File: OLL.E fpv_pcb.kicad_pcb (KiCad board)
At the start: 6 copper layers, 47.6 x 41.5 mm, 134 parts, among them J1 Micro_SD_Card, J10 Conn_01x05_Pin, J2 RC, J8 reciver, J9 TYPE-C-31-M-12, M1 M1 front left, M2 M2 front right, M3 M3 rear right, M4 m4 rear left, Q1 2N7002, Q2 SUD45P03-09, SW1 SW_SPST, SW2 SW_SPST, U1 MP2315GJ, U10 AON7410, U11 UCC27511ADBV, U12 AON7410, U13 BMP280, U14 STM32H753VITx, U15 USBLC6-2SC6, U3 MP2315GJ, U4 ICM-42688-P, U5 UCC27511ADBV, U6 ul_AON7410, U7 UCC27511ADBV, U8 AON7410, U9 UCC27511ADBV, Y2 8HMz

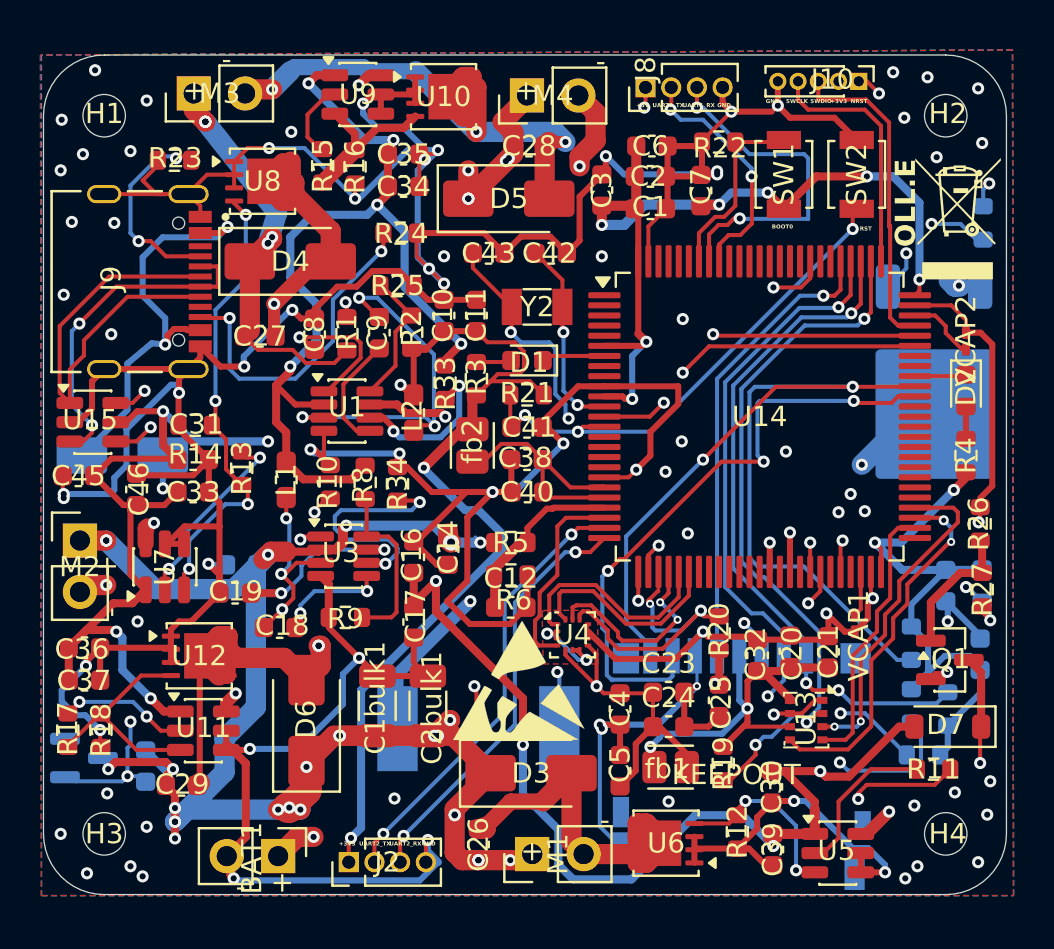
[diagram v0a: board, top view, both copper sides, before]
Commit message: latest scemetic
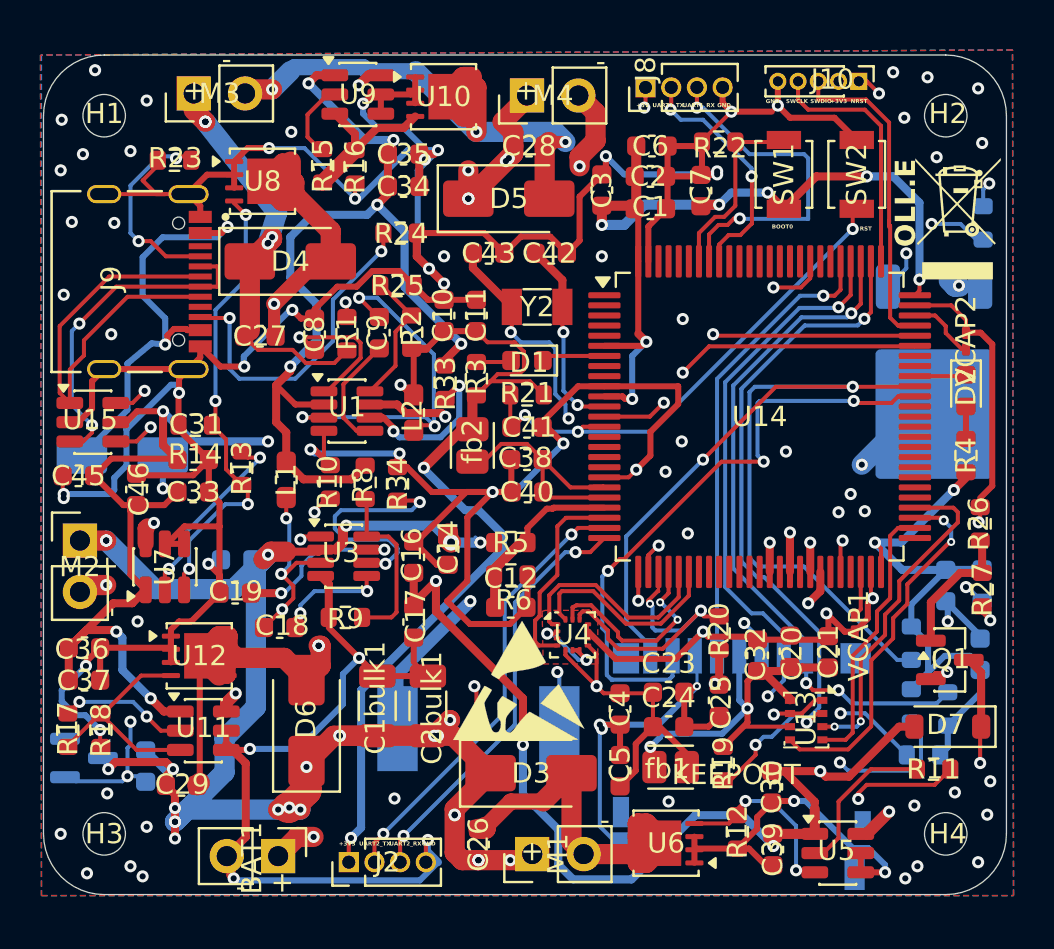
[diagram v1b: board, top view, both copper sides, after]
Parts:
- moved C15 0.35 mm to (142.9, 97.2)
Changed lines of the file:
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@@
 	(footprint "Capacitor_SMD:C_0603_1608Metric"
 		(layer "B.Cu")
-		(at 143.2 97.4 180)
+		(at 142.95 97.15 180)
 		(descr "Capacitor SMD 0603 (1608 Metric), square (rectangular) end terminal, IPC-7351 nominal, (Body size source: IPC-SM-782 page 76, https://www.pcb-3d.com/wordpress/wp-content/uploads/ipc-sm-782a_amendment_1_and_2.pdf), generated with kicad-footprint-generator")
 		(tags "capacitor")
@@
 		(start 151.85 81)
 		(end 151.85 82.15)
-		(width 0.2)
+		(width 0.4)
 		(layer "F.Cu")
 		(net 1)
@@
 		(start 141.15 79.655)
 		(end 140.57 79.075)
-		(width 0.2)
+		(width 0.3)
 		(layer "F.Cu")
 		(net 1)
@@
 		(start 142.825 77.465)
 		(end 143.49 76.8)
-		(width 0.2)
+		(width 0.3)
 		(layer "F.Cu")
 		(net 1)
@@
 		(start 151.85 82.15)
 		(end 153.2 83.5)
-		(width 0.2)
+		(width 0.4)
 		(layer "F.Cu")
 		(net 1)
@@
 		(start 143.49 76.8)
 		(end 144.55 76.8)
-		(width 0.2)
+		(width 0.3)
 		(layer "F.Cu")
 		(net 1)
@@
 		(start 141.15 80.2)
 		(end 141.15 79.655)
-		(width 0.2)
+		(width 0.3)
 		(layer "F.Cu")
 		(net 1)
@@
 		(start 140.57 79.03)
 		(end 141.485 78.115)
-		(width 0.2)
+		(width 0.3)
 		(layer "F.Cu")
 		(net 1)
@@
 	)
 	(segment
+		(start 173.8 112.6)
+		(end 175 112.6)
+		(width 0.3)
+		(layer "F.Cu")
+		(net 1)
+	)
+	(segment
 		(start 141.575 93.8)
 		(end 141.575 92.2)
@@
 		(start 142.825 77.465)
 		(end 142.825 78.765)
-		(width 0.2)
+		(width 0.3)
 		(layer "F.Cu")
 		(net 1)
@@
 		(start 151.975 77.1)
 		(end 152.7 77.1)
-		(width 0.2)
+		(width 0.4)
 		(layer "F.Cu")
 		(net 1)
@@
 	)
 	(segment
-		(start 173.8 112.6)
-		(end 175 112.6)
-		(width 0.3)
-		(layer "F.Cu")
-		(net 1)
-	)
-	(segment
 		(start 151.375 92.575)
 		(end 152.6 93.8)
@@
 		(start 164.175 79.8)
 		(end 163.3 80.675)
-		(width 0.2)
+		(width 0.3)
 		(layer "F.Cu")
 		(net 1)
@@
 	)
 	(segment
+		(start 163.3 82.4)
+		(end 163.3 80.675)
+		(width 0.3)
+		(layer "F.Cu")
+		(net 1)
+	)
+	(segment
 		(start 167.7 111.425)
 		(end 168.275 111.425)
@@
 	)
 	(segment
-		(start 163.3 80.675)
-		(end 163.3 82.4)
-		(width 0.2)
-		(layer "F.Cu")
-		(net 1)
-	)
-	(segment
 		(start 134.7 90.35)
 		(end 135.053052 90.35)
@@
 		(start 151.975 77.1)
 		(end 151.975 78.7)
-		(width 0.2)
+		(width 0.4)
 		(layer "F.Cu")
 		(net 1)
@@
 		(start 141.485 78.115)
 		(end 142.825 78.115)
-		(width 0.2)
+		(width 0.3)
 		(layer "F.Cu")
 		(net 1)
@@
 	)
 	(segment
-		(start 141.6 97.4)
-		(end 141.55 97.35)
-		(width 0.3)
-		(layer "B.Cu")
-		(net 1)
-	)
-	(segment
 		(start 136.9 93.1)
 		(end 136.9 93.7)
@@
 	)
 	(segment
+		(start 141.6 97.4)
+		(end 141.55 97.35)
+		(width 0.3)
+		(layer "B.Cu")
+		(net 1)
+	)
+	(segment
+		(start 142.175 97.15)
+		(end 141.925 97.4)
+		(width 0.3)
+		(layer "B.Cu")
+		(net 1)
+	)
+	(segment
 		(start 148.8 79.3)
 		(end 149 79.3)
@@
 	)
 	(segment
-		(start 142.425 97.4)
-		(end 141.6 97.4)
-		(width 0.3)
-		(layer "B.Cu")
-		(net 1)
-	)
-	(segment
 		(start 149.85 75.75)
 		(end 151.15 75.75)
@@
 	)
 	(segment
+		(start 141.925 97.4)
+		(end 141.6 97.4)
+		(width 0.3)
+		(layer "B.Cu")
+		(net 1)
+	)
+	(segment
 		(start 152.9 112.1)
 		(end 152 113)
@@
 	)
 	(segment
-		(start 142.8 98.6)
-		(end 144.5 96.9)
-		(width 1)
+		(start 139.9 109.425)
+		(end 139.9 110.1)
+		(width 0.4)
 		(layer "B.Cu")
 		(net 3)
 	)
 	(segment
-		(start 139.9 109.425)
-		(end 139.9 110.1)
-		(width 0.4)
+		(start 136.5 96.2)
+		(end 138.9 98.6)
+		(width 1)
 		(layer "B.Cu")
 		(net 3)
@@
 	)
 	(segment
-		(start 136.5 96.2)
-		(end 138.9 98.6)
-		(width 1)
-		(layer "B.Cu")
-		(net 3)
-	)
-	(segment
 		(start 139.8 107.5)
 		(end 139.375 107.5)
@@
 	)
 	(segment
-		(start 138.9 98.6)
-		(end 142.8 98.6)
-		(width 1)
-		(layer "B.Cu")
-		(net 3)
-	)
-	(segment
 		(start 178.15 83.35)
 		(end 178.45 83.65)
@@
 	)
 	(segment
+		(start 142.8 98.6)
+		(end 144.5 96.9)
+		(width 1)
+		(layer "B.Cu")
+		(net 3)
+	)
+	(segment
 		(start 144.95 80)
 		(end 144.48 81.52)
@@
 	)
 	(segment
+		(start 138.9 98.6)
+		(end 142.8 98.6)
+		(width 1)
+		(layer "B.Cu")
+		(net 3)
+	)
+	(segment
 		(start 136.6 107.2125)
 		(end 136.3375 106.95)
@@
 		(start 159.05 84.65)
 		(end 159.05 83.325)
-		(width 0.2)
+		(width 0.4)
 		(layer "F.Cu")
 		(net 19)
@@
 		(start 159.05 83.325)
 		(end 157.725 82)
-		(width 0.2)
+		(width 0.4)
 		(layer "F.Cu")
 		(net 19)
@@
 		(start 156.55 84.65)
 		(end 154.625 82.725)
-		(width 0.2)
+		(width 0.4)
 		(layer "F.Cu")
 		(net 20)
@@
 		(start 154.625 82.725)
 		(end 154.625 82)
-		(width 0.2)
+		(width 0.4)
 		(layer "F.Cu")
 		(net 20)
@@
 		(start 169.3 96.3)
 		(end 169.3 97.75)
-		(width 0.3)
+		(width 0.4)
 		(layer "F.Cu")
 		(net 62)
@@
 		(start 170.3 95.8)
 		(end 170.3 97.75)
-		(width 0.3)
+		(width 0.4)
 		(layer "F.Cu")
 		(net 63)
@@
 		(start 171.3 96.3)
 		(end 171.3 97.75)
-		(width 0.2)
+		(width 0.4)
 		(layer "F.Cu")
 		(net 64)
@@
 	)
 	(segment
-		(start 171.2 99.3)
-		(end 171.8 98.7)
-		(width 0.2)
+		(start 142.4375 104.22151)
+		(end 142.4375 104.65)
+		(width 0.6)
 		(layer "F.Cu")
 		(net 65)
 	)
 	(segment
-		(start 171.8 98.7)
-		(end 171.8 97.75)
-		(width 0.2)
+		(start 171.2 99.3)
+		(end 171.8 98.7)
+		(width 0.4)
 		(layer "F.Cu")
 		(net 65)
 	)
 	(segment
-		(start 142.4375 104.22151)
-		(end 142.4375 104.65)
+		(start 142.9 103.75901)
+		(end 142.4375 104.22151)
 		(width 0.6)
 		(layer "F.Cu")
@@
 	)
 	(segment
-		(start 142.9 103.75901)
-		(end 142.4375 104.22151)
-		(width 0.6)
+		(start 171.8 98.7)
+		(end 171.8 97.75)
+		(width 0.4)
 		(layer "F.Cu")
 		(net 65)
